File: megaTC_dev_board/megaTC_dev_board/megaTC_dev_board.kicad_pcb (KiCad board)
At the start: 4 copper layers, 72.8 x 36.5 mm, 35 parts, among them J1 Conn_01x08_Pin, J2 Conn_01x08_Pin, J3 Conn_01x08_Pin, U1 LTC2984CLX-PBF, U2 TPD4E1B06DCKR, U3 TPD4E1B06DCKR, U4 TPD4E1B06DCKR, U5 TPD4E1B06DCKR, U6 TPD4E1B06DCKR

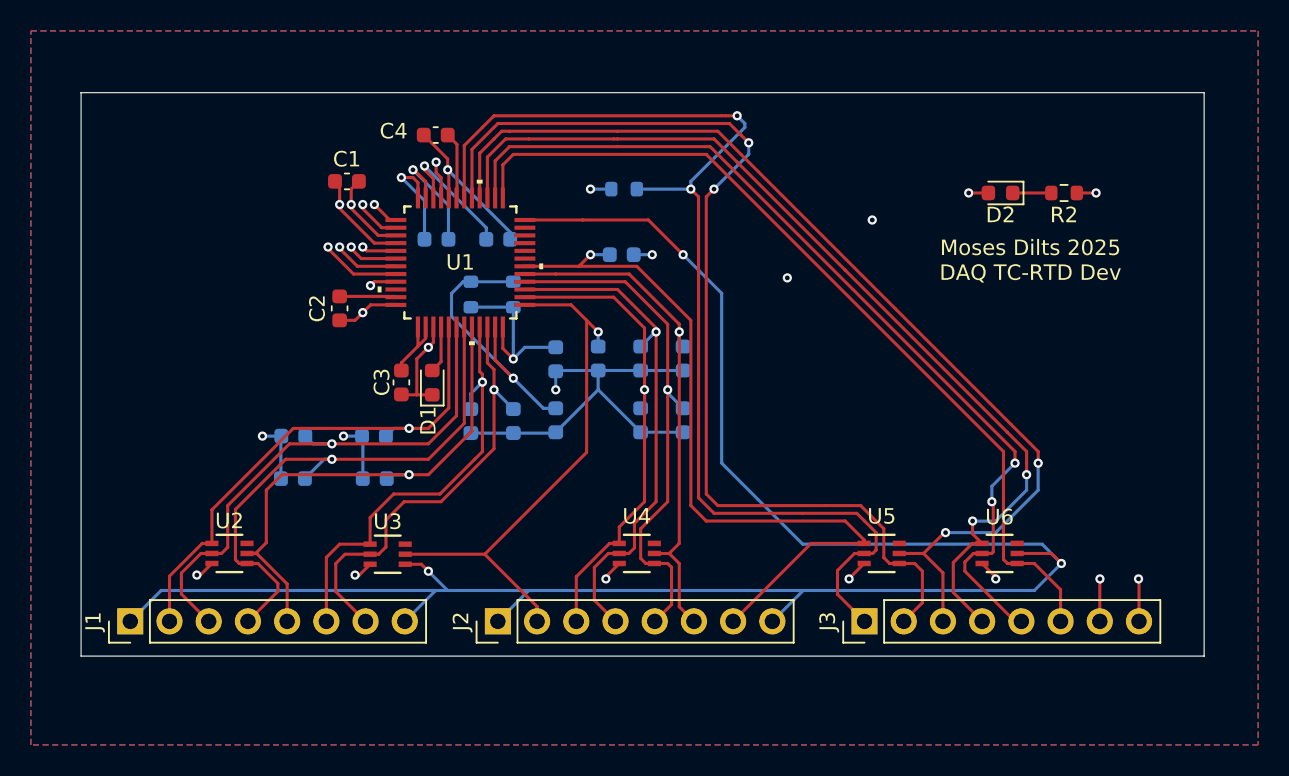
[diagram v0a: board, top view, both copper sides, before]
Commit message: routing updates
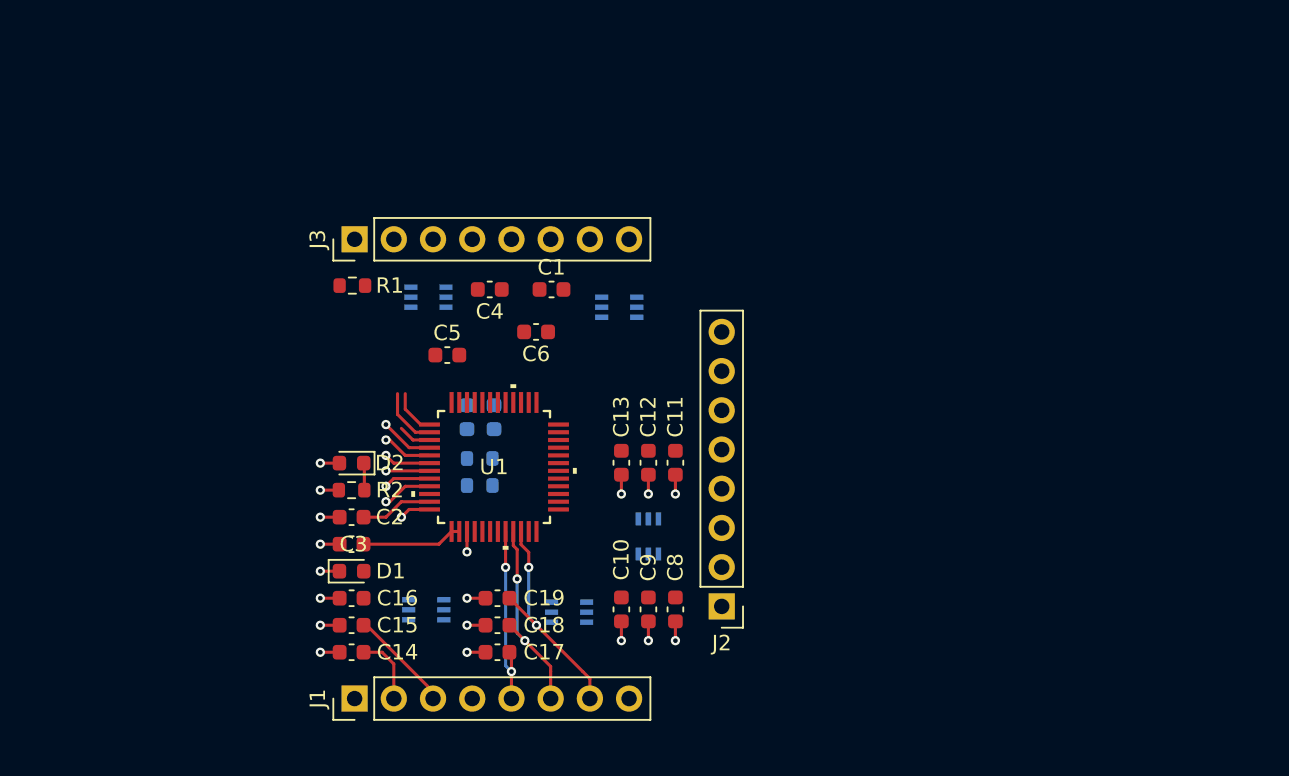
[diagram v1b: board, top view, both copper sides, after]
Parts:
- C10, C11, C12, C13, C14, C15, C16, C17, C18, C19, C5, C6, C8, C9, R1: moved to F.Cu
- U2, U3, U4, U5, U6: moved to B.Cu
- moved R2 50.0 mm to (142.8, 114.5), turned to 0 degrees
- moved D2 45.5 mm to (142.8, 112.8)
- moved J3 41.3 mm to (143.0, 98.2)
- moved U5 33.7 mm to (147.8, 102.0)
- moved U6 29.3 mm to (160.1, 102.6)
- moved R1 18.7 mm to (142.8, 101.2)
- moved C8 17.0 mm to (163.8, 122.2)
- moved C10 16.3 mm to (160.2, 122.2)
- moved J1 15.4 mm to (143.0, 128.0)
- moved C1 15.0 mm to (155.7, 101.5)
- moved J2 14.5 mm to (166.8, 122.0), turned to 180 degrees
- moved C14 14.1 mm to (142.8, 125.0)
- moved C17 13.8 mm to (152.2, 125.0)
- moved C2 13.5 mm to (142.8, 116.2), turned to 0 degrees
- moved C13 13.5 mm to (160.2, 112.7), turned to -90 degrees
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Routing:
- net COMMON: track 127.4 -> 0.00 mm, vias 3 -> 0
- net RESET_LOW: track 72.6 -> 0.00 mm, vias 2 -> 0
- net CS_LOW: track 67.1 -> 0.00 mm, vias 2 -> 0
- net SDI: track 66.4 -> 0.00 mm, vias 2 -> 0
- net SDO: track 61.9 -> 0.00 mm, vias 2 -> 0
- net SCK: track 59.5 -> 0.00 mm, vias 2 -> 0
- net INTERRUPT: track 56.4 -> 0.00 mm
- net CH15: track 49.5 -> 0.00 mm, vias 1 -> 0
- net GND: track 84.1 -> 37.6 mm
- net CH4: track 35.6 -> 0.00 mm, vias 1 -> 0
- net CH10: track 35.2 -> 0.00 mm, vias 1 -> 0
- net CH13: track 34.1 -> 0.00 mm, vias 1 -> 0
- net CH14: track 33.5 -> 0.00 mm, vias 1 -> 0
- net CH12: track 32.9 -> 0.00 mm, vias 1 -> 0
- net CH11: track 31.1 -> 0.00 mm, vias 1 -> 0
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- removed copper zone on B.Cu, net GND
- removed copper zone on F.Cu, net GND
- removed copper zone on In2.Cu, net GND
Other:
- board outline removed
- board text removed: "Moses Dilts 2025 DAQ TC-RTD Dev"

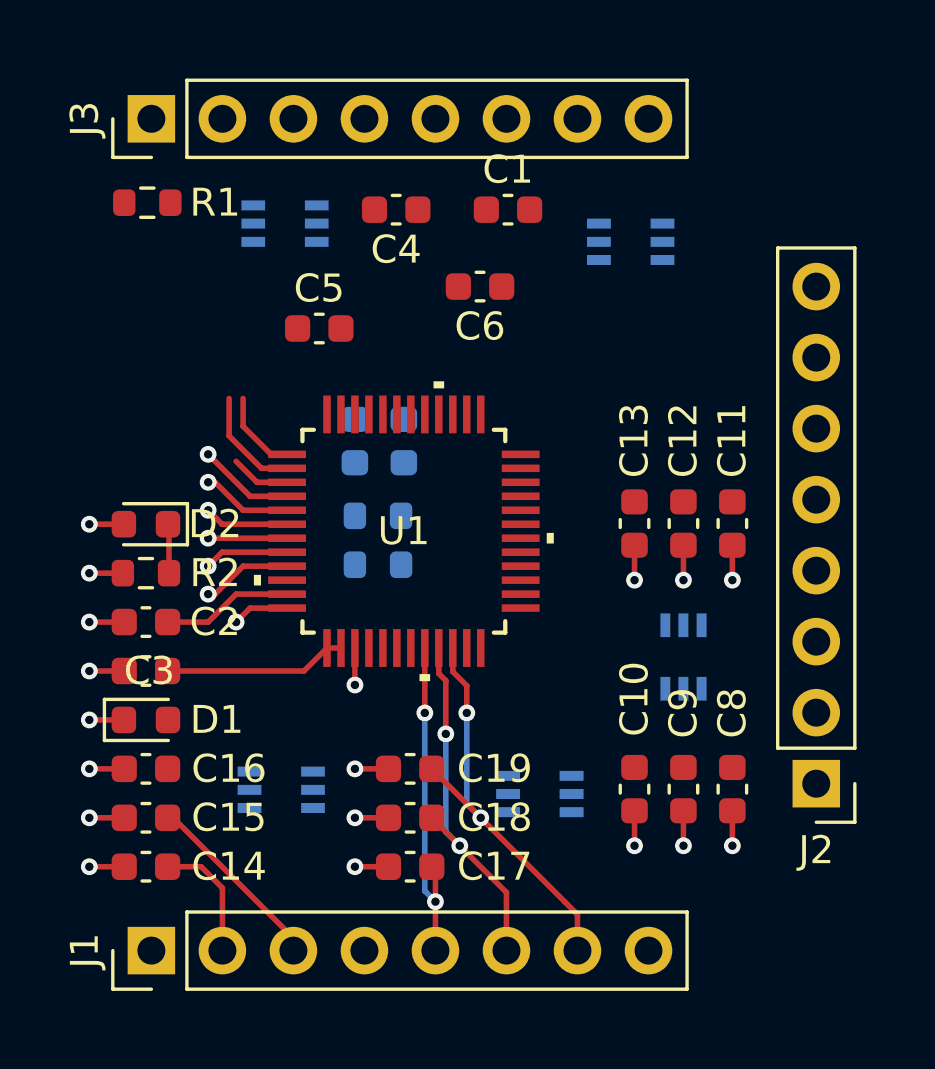
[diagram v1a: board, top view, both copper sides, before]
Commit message: routing progress
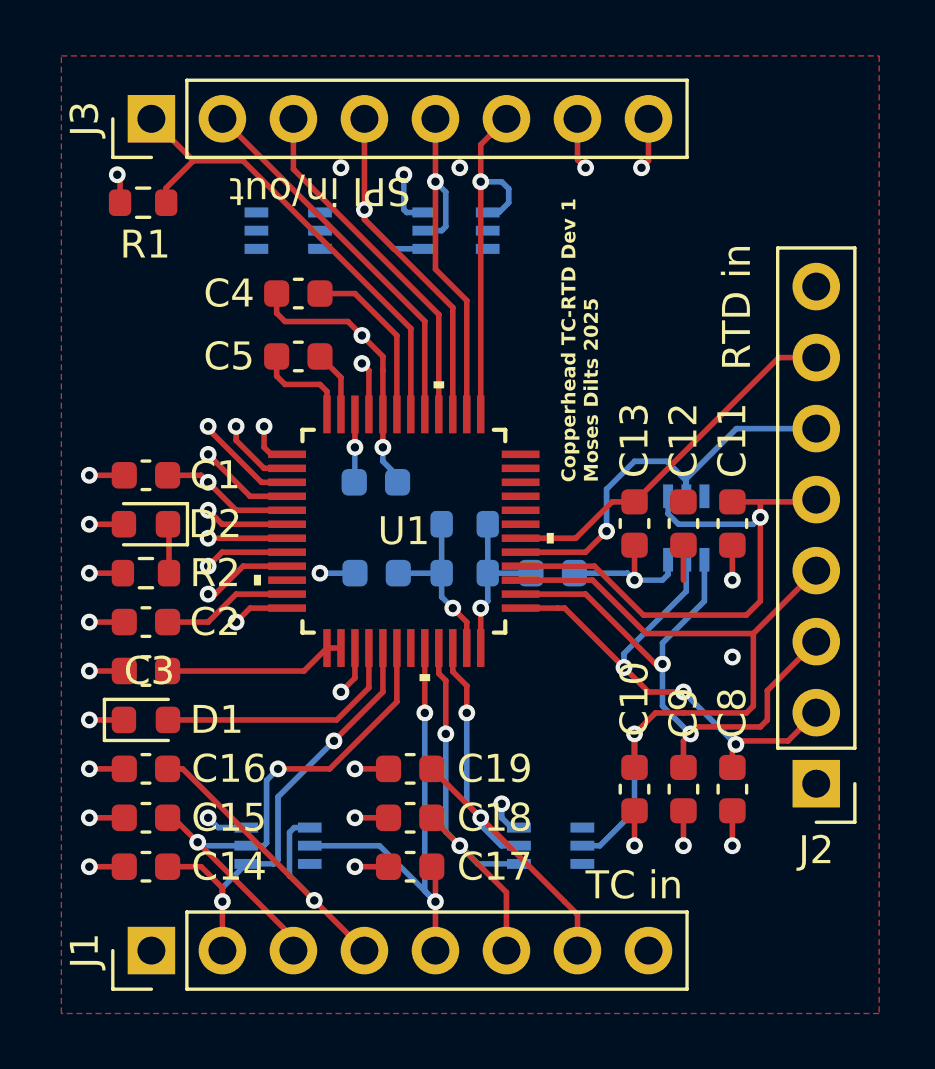
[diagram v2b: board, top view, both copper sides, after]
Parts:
- C6: moved to B.Cu
- moved C1 16.1 mm to (142.8, 111.0)
- moved C6 7.93 mm to (151.0, 111.2), turned to 0 degrees
- moved C21 7.12 mm to (157.3, 114.5), turned to 0 degrees
- moved U6 6.26 mm to (153.9, 102.2)
- moved C20 4.79 mm to (151.0, 114.5), turned to 180 degrees
- moved U4 4.61 mm to (162.1, 112.9), turned to 90 degrees
- moved C4 4.61 mm to (148.2, 104.5)
- moved R3 3.11 mm to (154.2, 114.5)
- moved R4 3.11 mm to (154.2, 112.8)
- moved U2 2.00 mm to (147.5, 124.2)
- moved U3 1.89 mm to (157.2, 124.2), turned to 0 degrees
- moved C5 1.25 mm to (148.2, 106.8)
- moved U5 0.27 mm to (147.9, 102.2)
- moved R1 0.15 mm to (142.7, 101.2)
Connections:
- U3 pad 5: CH10 -> CH12
- U4 pad 2: CH12 -> CH10
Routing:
- net CH12: track 0.00 -> 25.9 mm, vias 0 -> 1
- net GND: track 37.6 -> 61.6 mm, vias 21 -> 32
- net CH11: track 0.00 -> 21.2 mm, vias 0 -> 2
- net CH13: track 0.00 -> 20.3 mm, vias 0 -> 1
- net CH10: track 0.00 -> 18.7 mm, vias 0 -> 3
- net RESET_LOW: track 0.00 -> 17.4 mm
- net CH14: track 0.00 -> 15.0 mm, vias 0 -> 1
- net SDO: track 0.00 -> 14.8 mm, vias 0 -> 1
- net SCK: track 0.00 -> 13.6 mm, vias 0 -> 1
- net CS_LOW: track 0.00 -> 13.6 mm
- net INTERRUPT: track 0.00 -> 13.5 mm, vias 0 -> 1
- net CH4: track 0.00 -> 13.3 mm, vias 0 -> 1
- net CH15: track 0.00 -> 13.2 mm
- net SDI: track 0.00 -> 12.7 mm
- net CH3: track 6.73 -> 19.3 mm, vias 0 -> 2
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- added copper zone on F.Cu, net GND
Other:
- board text added: "Copperhead TC-RTD Dev 1 Moses Dilts 2025"
- board text added: "RTD in"
- board text added: "SPI in/out"
- board text added: "TC in"

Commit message: routing that is less spahghetti-like wait is that how you spell spahghetti idk i hope so because im committing it rn so it better be right
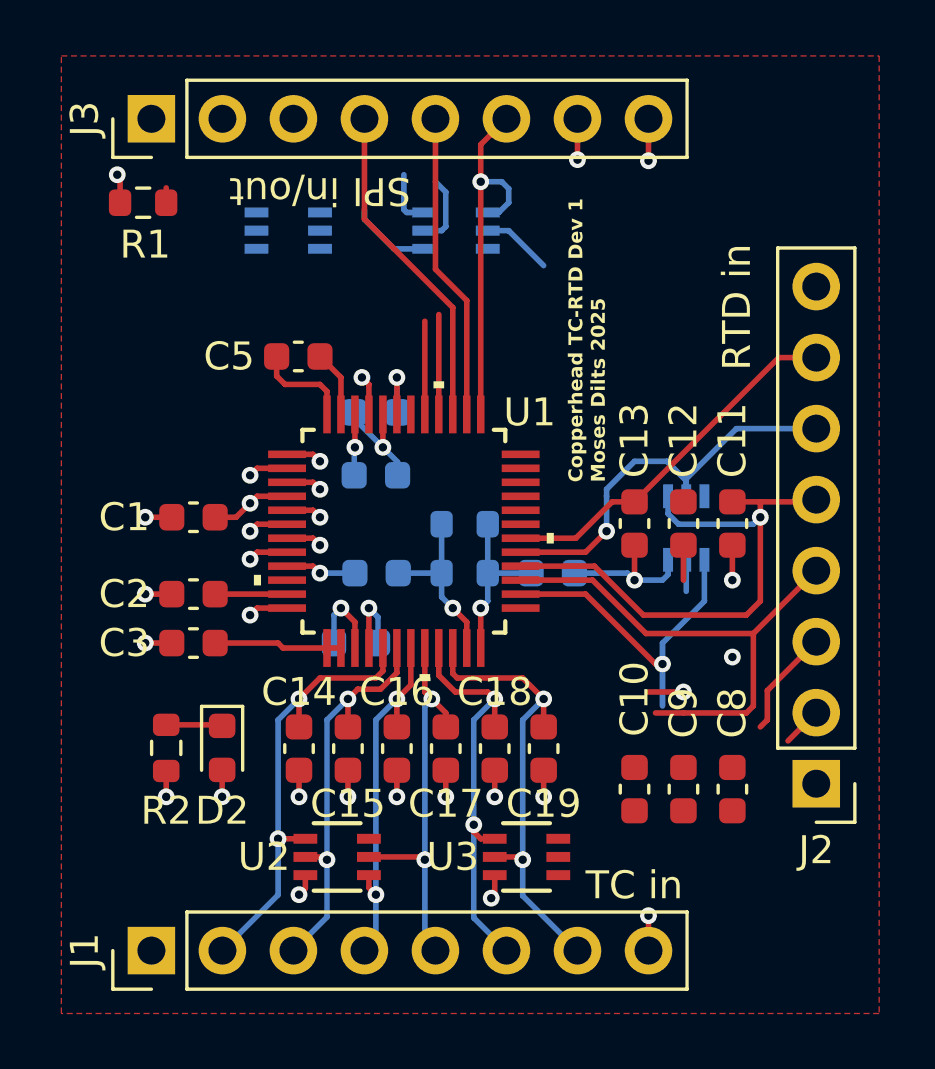
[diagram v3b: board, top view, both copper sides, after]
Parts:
- C4, D1: moved to B.Cu
- U2, U3: moved to F.Cu
- moved C16 9.00 mm to (151.8, 120.8), turned to -90 degrees
- moved D2 8.45 mm to (145.5, 120.8), turned to -90 degrees
- moved D1 8.00 mm to (150.3, 117.0)
- moved C15 7.64 mm to (150.0, 120.8), turned to -90 degrees
- moved C14 6.92 mm to (148.2, 120.8), turned to -90 degrees
- moved R2 6.29 mm to (143.5, 120.8), turned to 90 degrees
- moved C4 5.08 mm to (151.0, 108.8)
- moved C19 4.83 mm to (157.0, 120.8), turned to -90 degrees
- moved C17 4.41 mm to (153.5, 120.8), turned to -90 degrees
- moved C18 3.91 mm to (155.2, 120.8), turned to -90 degrees
- moved C1 2.27 mm to (144.5, 112.5), turned to 180 degrees
- moved U2 2.15 mm to (149.6, 124.6)
- moved C2 1.97 mm to (144.5, 115.2)
- moved C3 1.97 mm to (144.5, 117.0)
- moved U3 0.95 mm to (156.4, 124.6)
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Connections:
- J1 pad 8: COMMON -> GND
- J2 pad 1: COMMON -> GND
- J2 pad 8: COMMON -> GND
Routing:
- net GND: track 61.6 -> 40.0 mm, vias 32 -> 25
- net RESET_LOW: track 17.4 -> 0.53 mm
- net CH10: track 18.7 -> 3.81 mm, vias 3 -> 1
- net CS_LOW: track 13.6 -> 3.33 mm
- net SDI: track 12.7 -> 3.57 mm
- net +5V: track 19.6 -> 12.0 mm, vias 9 -> 8
- net CH12: track 25.9 -> 18.5 mm, vias 1 -> 0
- net CH1: track 9.09 -> 2.81 mm, vias 0 -> 1
- net CH11: track 21.2 -> 15.8 mm, vias 2 -> 1
- net CH3: track 19.3 -> 15.1 mm
- net Net-(U1-LDO): track 6.19 -> 2.58 mm, vias 0 -> 1
- net CH5: track 17.6 -> 14.4 mm
- net COMMON: track 0.00 -> 2.52 mm
- net Net-(U1-VREF_BYP): track 4.69 -> 2.57 mm
- net Net-(U1-VREFOUT): track 6.54 -> 4.57 mm
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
